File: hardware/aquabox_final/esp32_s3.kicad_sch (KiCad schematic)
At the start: 2 parts, among them J3 TFT - 1.8{dblquote} SPI, U2 ESP32-S3-DEVKITC-1-N16R8V

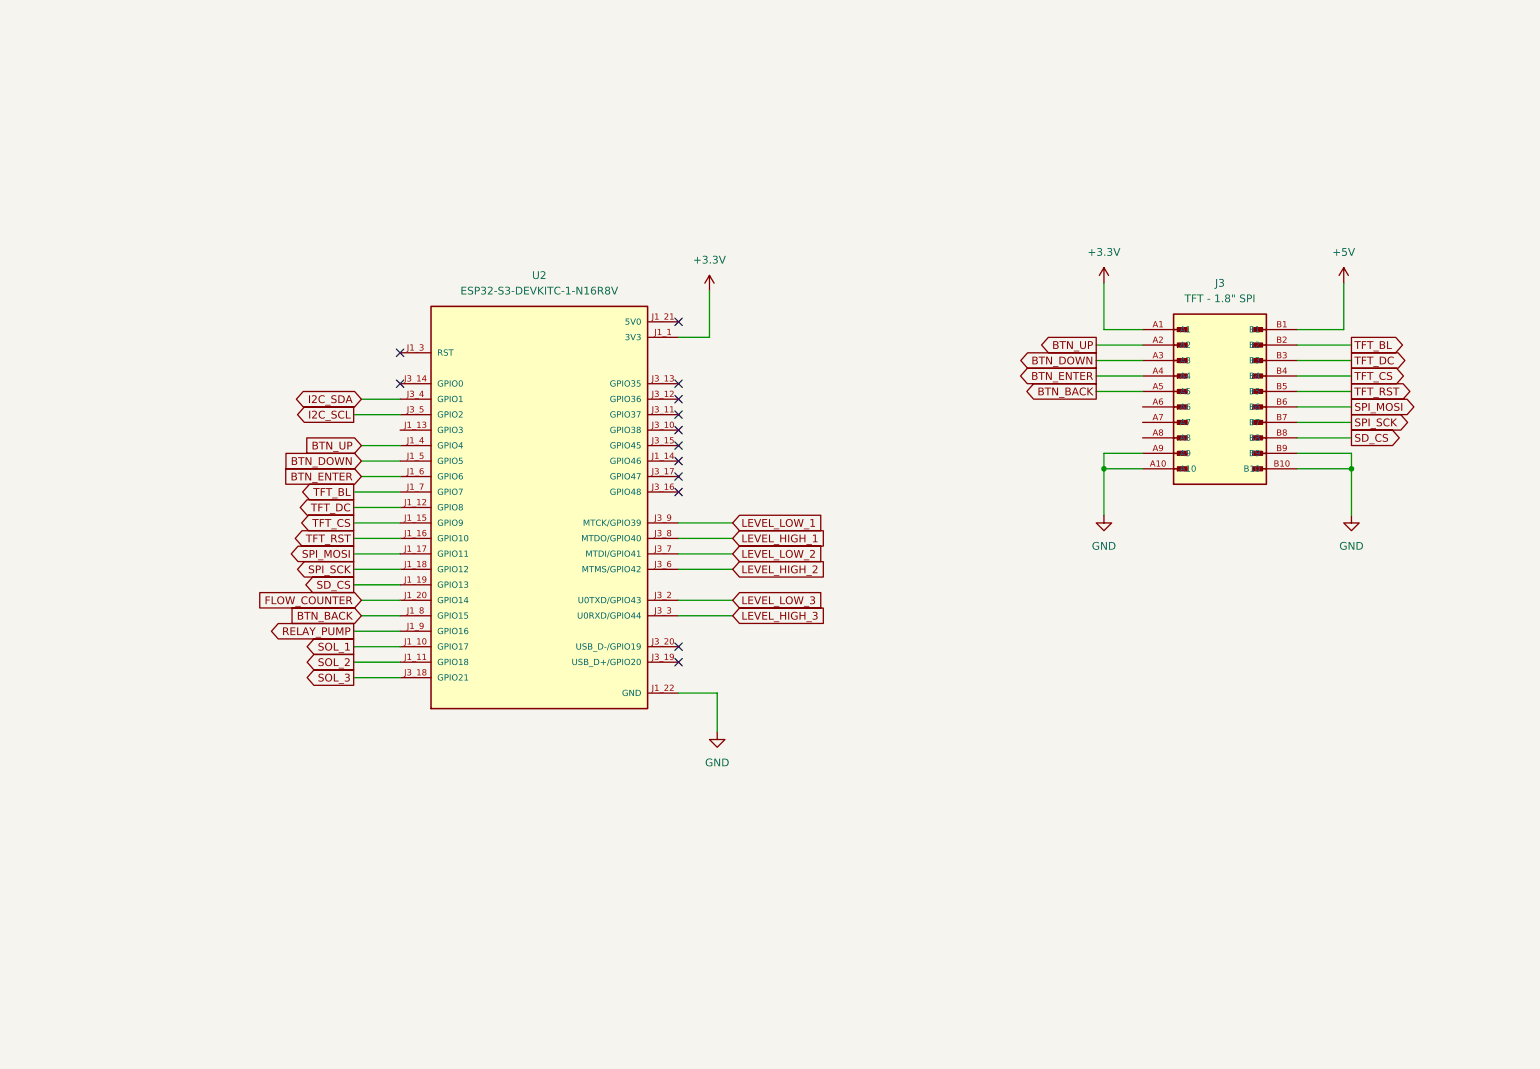
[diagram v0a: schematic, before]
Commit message: Atualização
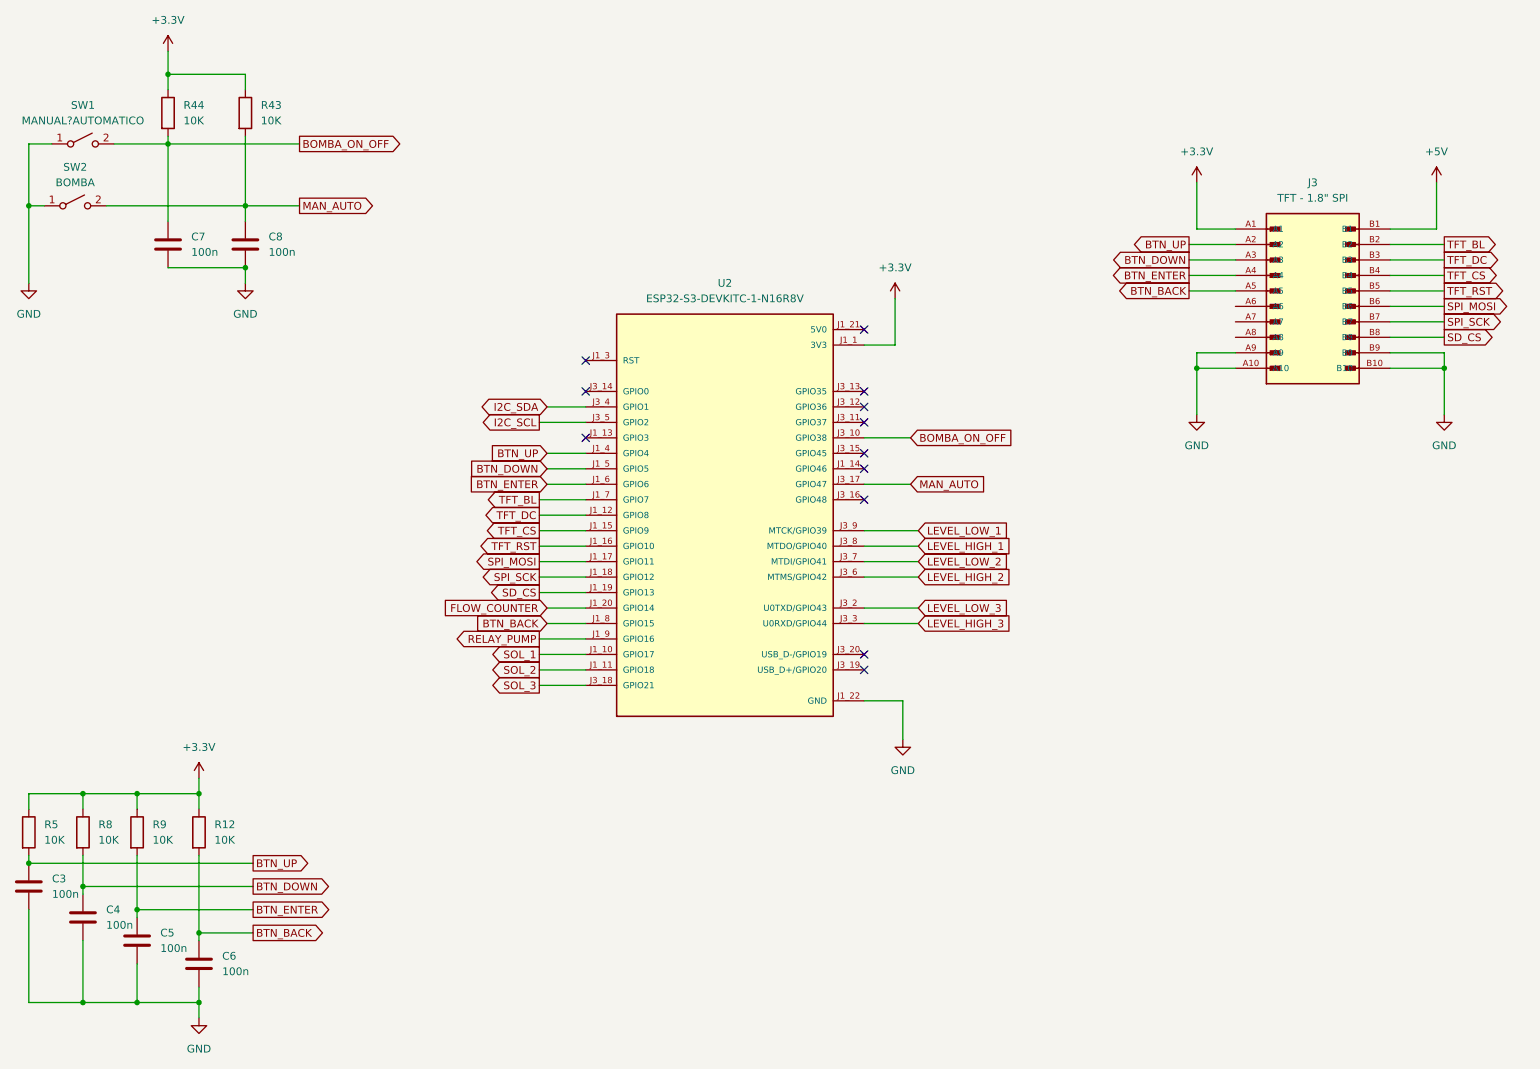
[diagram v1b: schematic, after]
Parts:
- added C3, C4, C5, C6, C7, C8: 100n, symbol Device:C
- added R12, R43, R44, R5, R8, R9: 10K, symbol Device:R
- added SW1: MANUAL?AUTOMATICO, symbol Switch:SW_SPST
- added SW2: BOMBA, symbol Switch:SW_SPST
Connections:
- net +3.3V: now also R12.1, R43.1, R44.1, R5.1, R8.1, R9.1
- net BTN_BACK: now also C6.1, R12.2
- net BTN_DOWN: now also C4.1, R8.2
- net BTN_ENTER: now also C5.1, R9.2
- net BTN_UP: now also C3.1, R5.2
- net GND: now also C3.2, C4.2, C5.2, C6.2, C7.2, C8.2, SW1.1 (A), SW2.1 (A)
- net BOMBA_ON_OFF: now reaches U2.J3_10 (GPIO38)
- net BOMBA_ON_OFF: now also C7.1, R44.2, SW1.2 (B)
- net MAN_AUTO: now reaches U2.J3_17 (GPIO47)
- net MAN_AUTO: now also C8.1, R43.2, SW2.2 (B)
- no-connect marks 13 -> 12
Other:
- moved on the sheet: J3, U2
